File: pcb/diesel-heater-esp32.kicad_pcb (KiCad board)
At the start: 2 copper layers, 60 x 45 mm, 29 parts, among them J1 5V Power, J10 Fan Motor, J11 Glow Plug, J12 Oil Pump, J2 ESP32 Left, J3 Hall Sensor, J4 Buttons, J5 Battery Mon, J6 ESP32 Right, J7 OLED, J8 NTC50K Room Temperatire, J9 NTC50K Outlet Temperatire

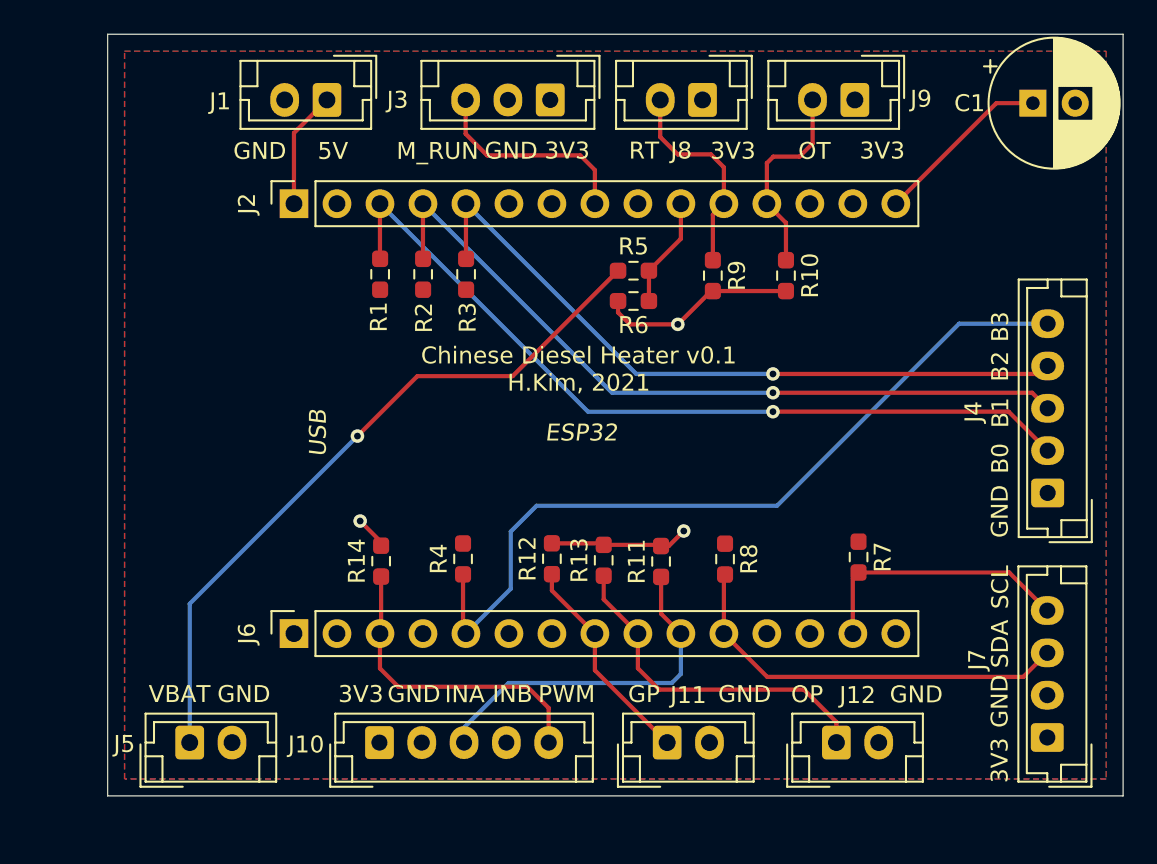
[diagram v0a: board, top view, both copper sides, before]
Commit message: releasing pcb 0.1
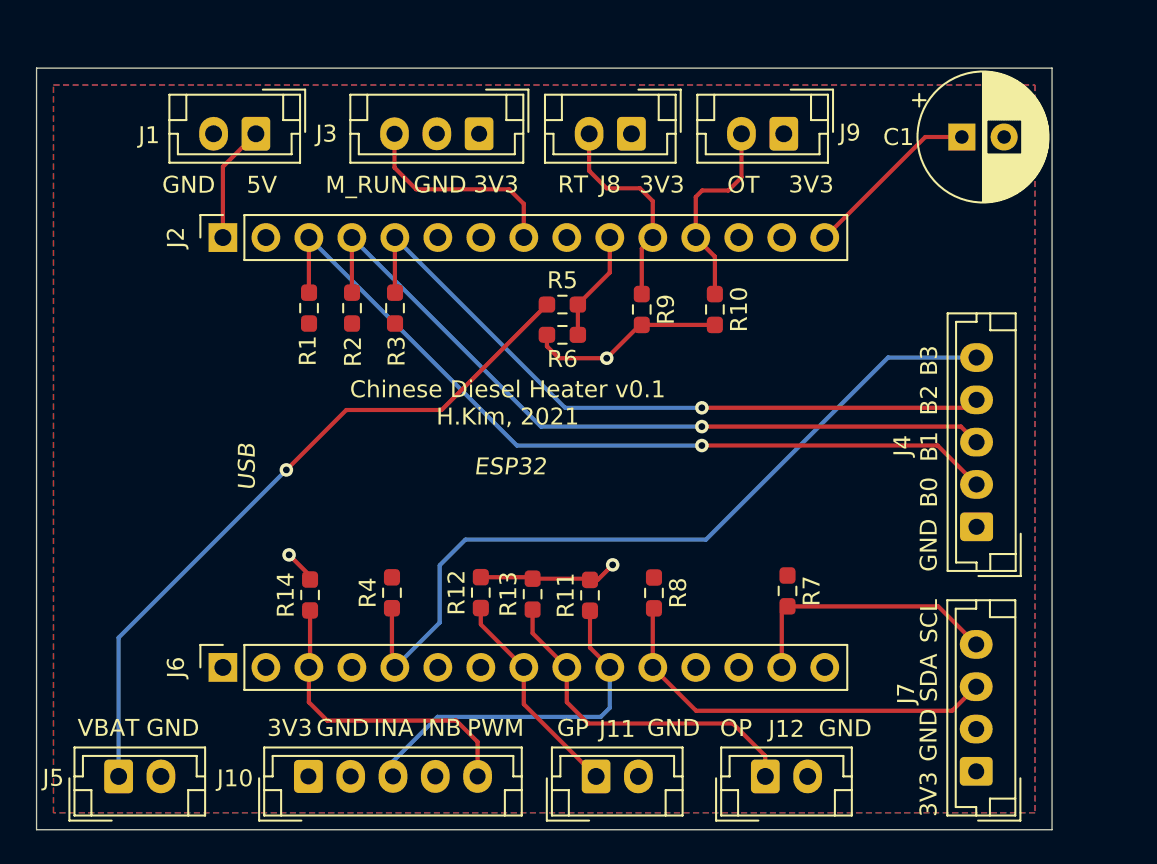
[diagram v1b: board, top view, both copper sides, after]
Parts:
- moved C1 4.65 mm to (164.7, 74.0)
- moved J4 4.65 mm to (165.6, 97.0)
- moved R1 4.65 mm to (126.2, 84.1)
- moved R10 4.65 mm to (150.1, 84.2)
- moved R11 4.65 mm to (142.8, 101.0)
- moved R2 4.65 mm to (128.7, 84.1)
- moved R5 4.65 mm to (141.1, 83.9)
- moved R6 4.65 mm to (141.1, 85.7)
- moved R8 4.65 mm to (146.5, 100.9)
- moved R9 4.65 mm to (145.8, 84.2)
- moved J1 4.65 mm to (123.0, 73.8)
- moved J2 4.65 mm to (121.1, 79.9)
- moved J5 4.65 mm to (114.9, 111.8)
- moved J6 4.65 mm to (121.1, 105.3)
- moved REF** 4.65 mm to (119.3, 91.0)
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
